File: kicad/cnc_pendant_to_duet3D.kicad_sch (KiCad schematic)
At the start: 9 parts, among them J1 Conn_01x04_Male, J2 DA15_Socket_MountingHoles, U1 Sparkfun_Pro_Micro

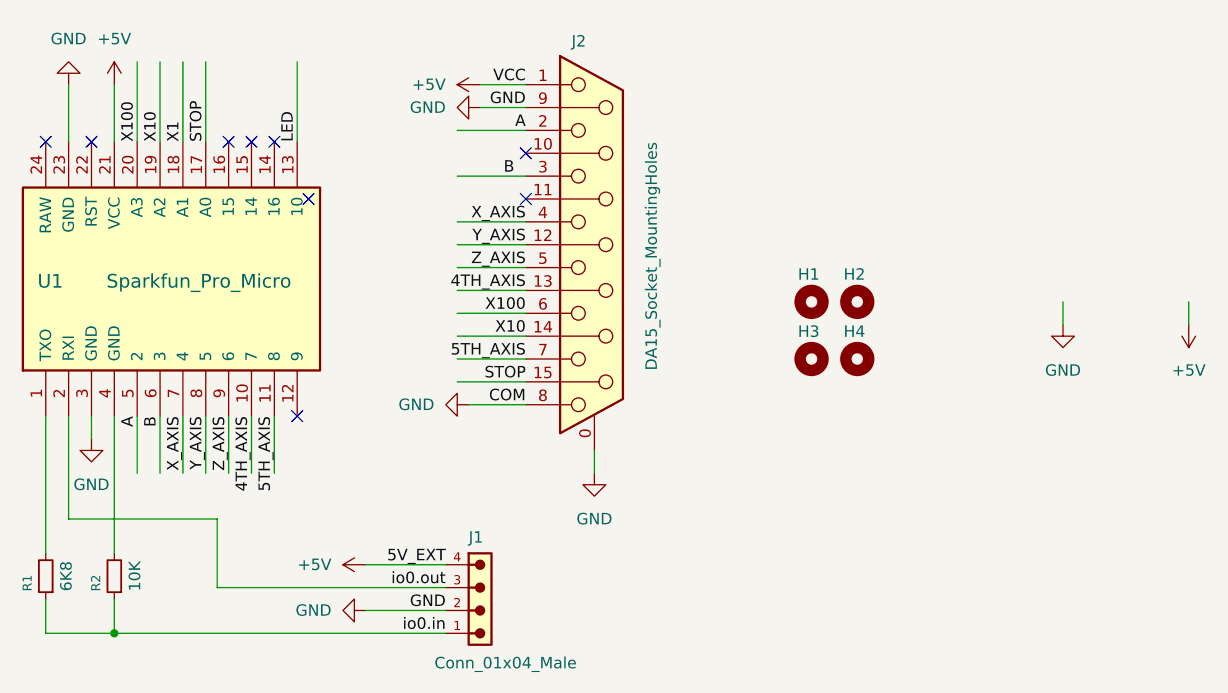
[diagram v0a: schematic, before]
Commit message: renaming
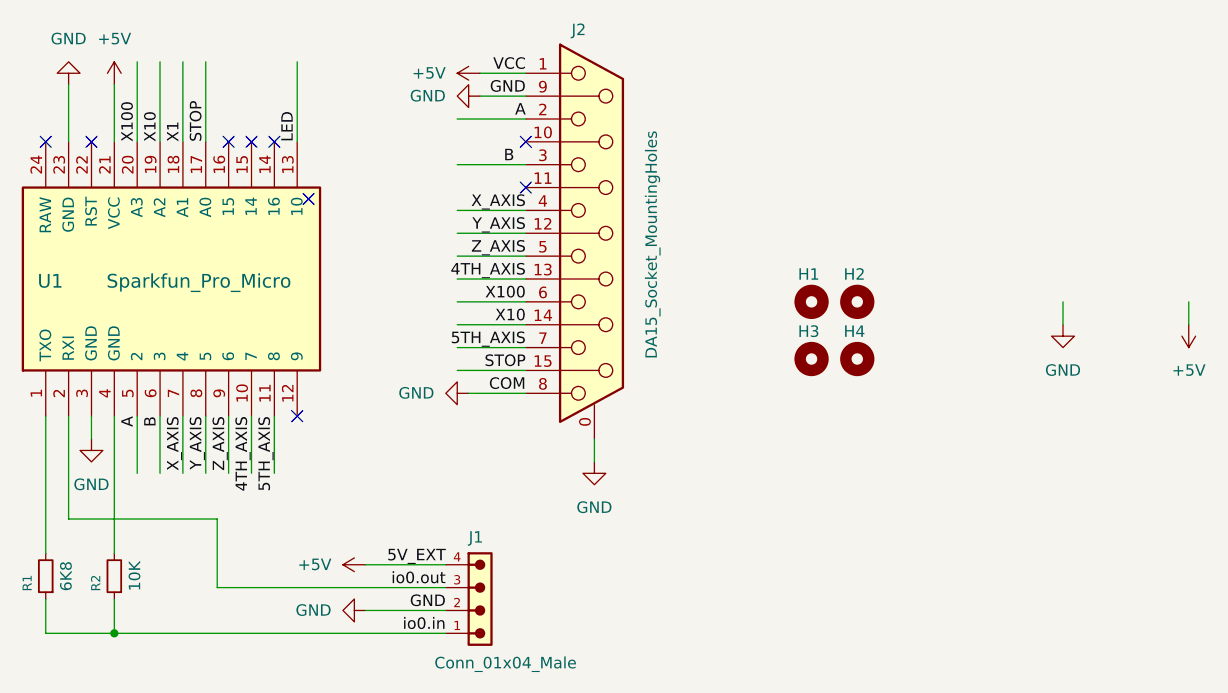
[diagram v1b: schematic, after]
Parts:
- J1: footprint cnc_pendant_to_duet3D:61900411021 -> cnc_pendant_to_duet3d:61900411021
- U1: footprint cnc_pendant_to_duet3D:Sparkfun_Pro_Micro -> cnc_pendant_to_duet3d:Sparkfun_Pro_Micro; symbol cnc_pendant_to_duet3D:Sparkfun_Pro_Micro -> cnc_pendant_to_duet3d:Sparkfun_Pro_Micro
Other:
- moved on the sheet: J2
